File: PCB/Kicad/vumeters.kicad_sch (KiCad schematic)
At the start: 80 parts

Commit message: update elements WIP
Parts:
- D1, D10, D11, D12, D13, D14, D15, D16, D17, D18, D19, D2, D20, D21, D22, D23, D24, D25, D26, D27, D28, D29, D3, D30, D31, D32, D33, D34, D35, D36, D37, D38, D39, D4, D40, D5, D6, D7, D8, D9: renamed from D?; symbol Traktorino-rescue:LED_ALT-Device -> Device:LED_Filled
- gave numbers to parts that had none: 40
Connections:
- net GND: now also D1.1 (K), D10.1 (K), D11.1 (K), D12.1 (K), D13.1 (K), D14.1 (K), D15.1 (K), D16.1 (K), D17.1 (K), D18.1 (K), D19.1 (K), D2.1 (K), D20.1 (K), D21.1 (K), D22.1 (K), D23.1 (K), D24.1 (K), D25.1 (K), D26.1 (K), D27.1 (K), D28.1 (K), D29.1 (K), D3.1 (K), D30.1 (K), D31.1 (K), D32.1 (K), D33.1 (K), D34.1 (K), D35.1 (K), D36.1 (K), D37.1 (K), D38.1 (K), D39.1 (K), D4.1 (K), D40.1 (K), D5.1 (K), D6.1 (K), D7.1 (K), D8.1 (K), D9.1 (K)
- net at R1.2: now also D1.2 (A)
- net at R2.2: now also D2.2 (A)
- net at R3.2: now also D3.2 (A)
- net at R4.2: now also D4.2 (A)
- net at R5.2: now also D5.2 (A)
- net at R6.2: now also D6.2 (A)
- net at R7.2: now also D7.2 (A)
- net at R8.2: now also D8.2 (A)
- net at R16.2: now also D16.2 (A)
- net at R15.2: now also D15.2 (A)
- net at R14.2: now also D14.2 (A)
- net at R13.2: now also D13.2 (A)
- net at R12.2: now also D12.2 (A)
- net at R11.2: now also D11.2 (A)
- net at R10.2: now also D10.2 (A)
- net at R9.2: now also D9.2 (A)
- net at R24.2: now also D24.2 (A)
- net at R23.2: now also D23.2 (A)
- net at R22.2: now also D22.2 (A)
- net at R21.2: now also D21.2 (A)
- net at R20.2: now also D20.2 (A)
- net at R19.2: now also D19.2 (A)
- net at R18.2: now also D18.2 (A)
- net at R17.2: now also D17.2 (A)
- net at R32.2: now also D32.2 (A)
- net at R31.2: now also D31.2 (A)
- net at R30.2: now also D30.2 (A)
- net at R29.2: now also D29.2 (A)
- net at R28.2: now also D28.2 (A)
- net at R27.2: now also D27.2 (A)
- net at R26.2: now also D26.2 (A)
- net at R25.2: now also D25.2 (A)
- net at R40.2: now also D40.2 (A)
- net at R39.2: now also D39.2 (A)
- net at R38.2: now also D38.2 (A)
- net at R37.2: now also D37.2 (A)
- net at R36.2: now also D36.2 (A)
- net at R35.2: now also D35.2 (A)
- net at R34.2: now also D34.2 (A)
- net at R33.2: now also D33.2 (A)

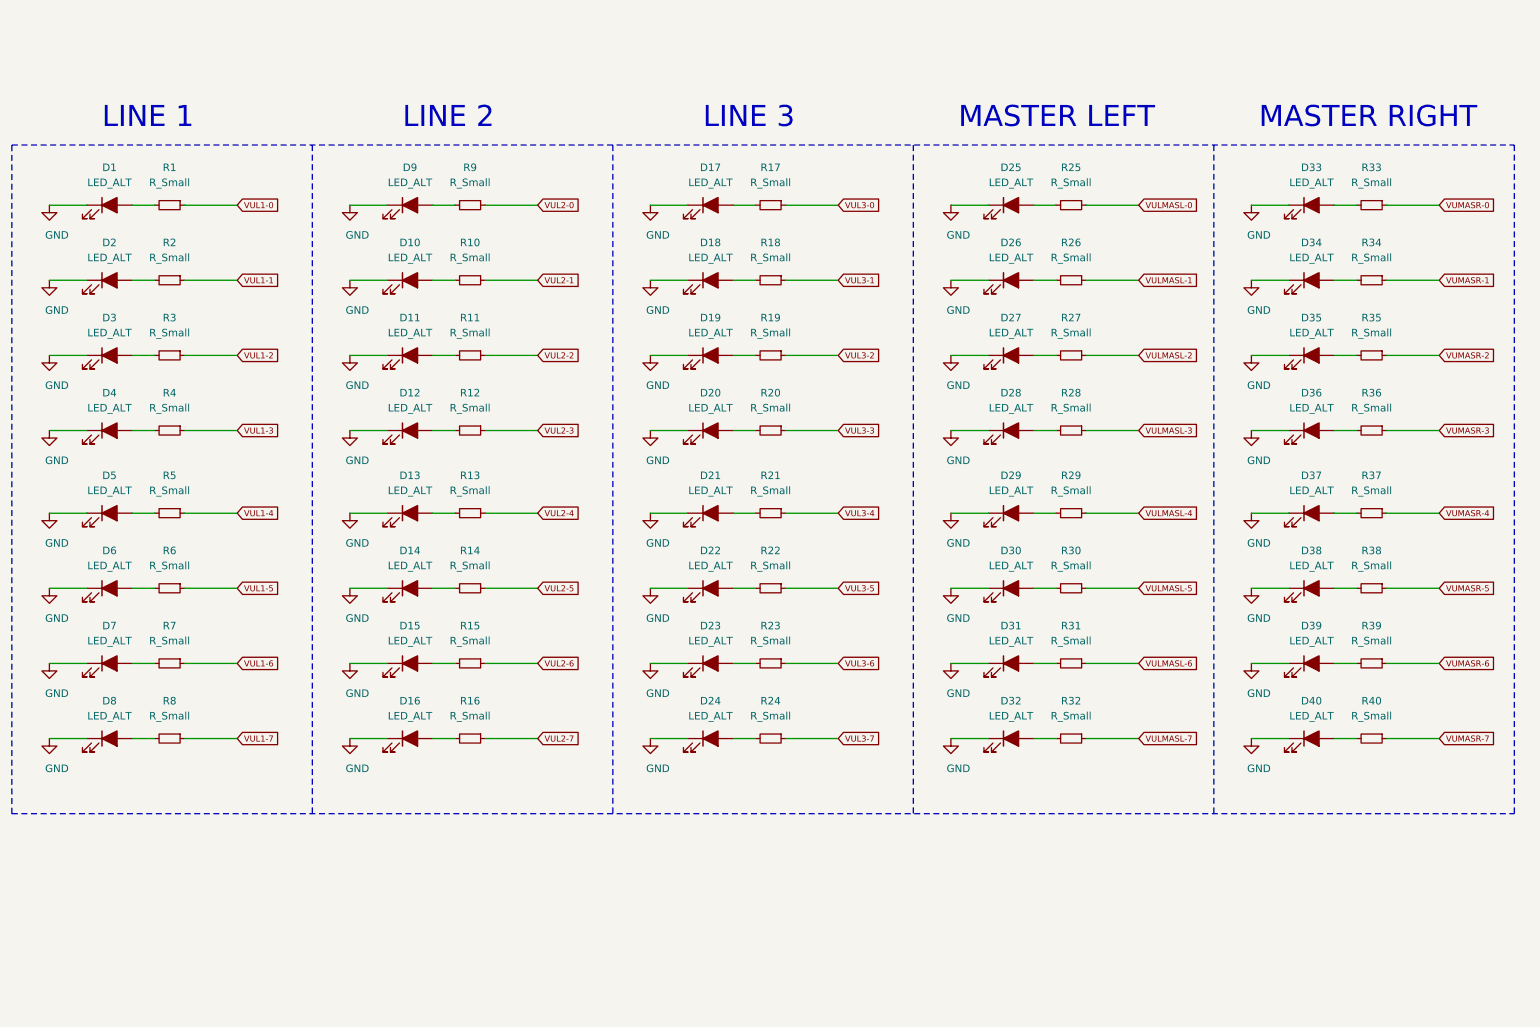
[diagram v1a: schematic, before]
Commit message: progress
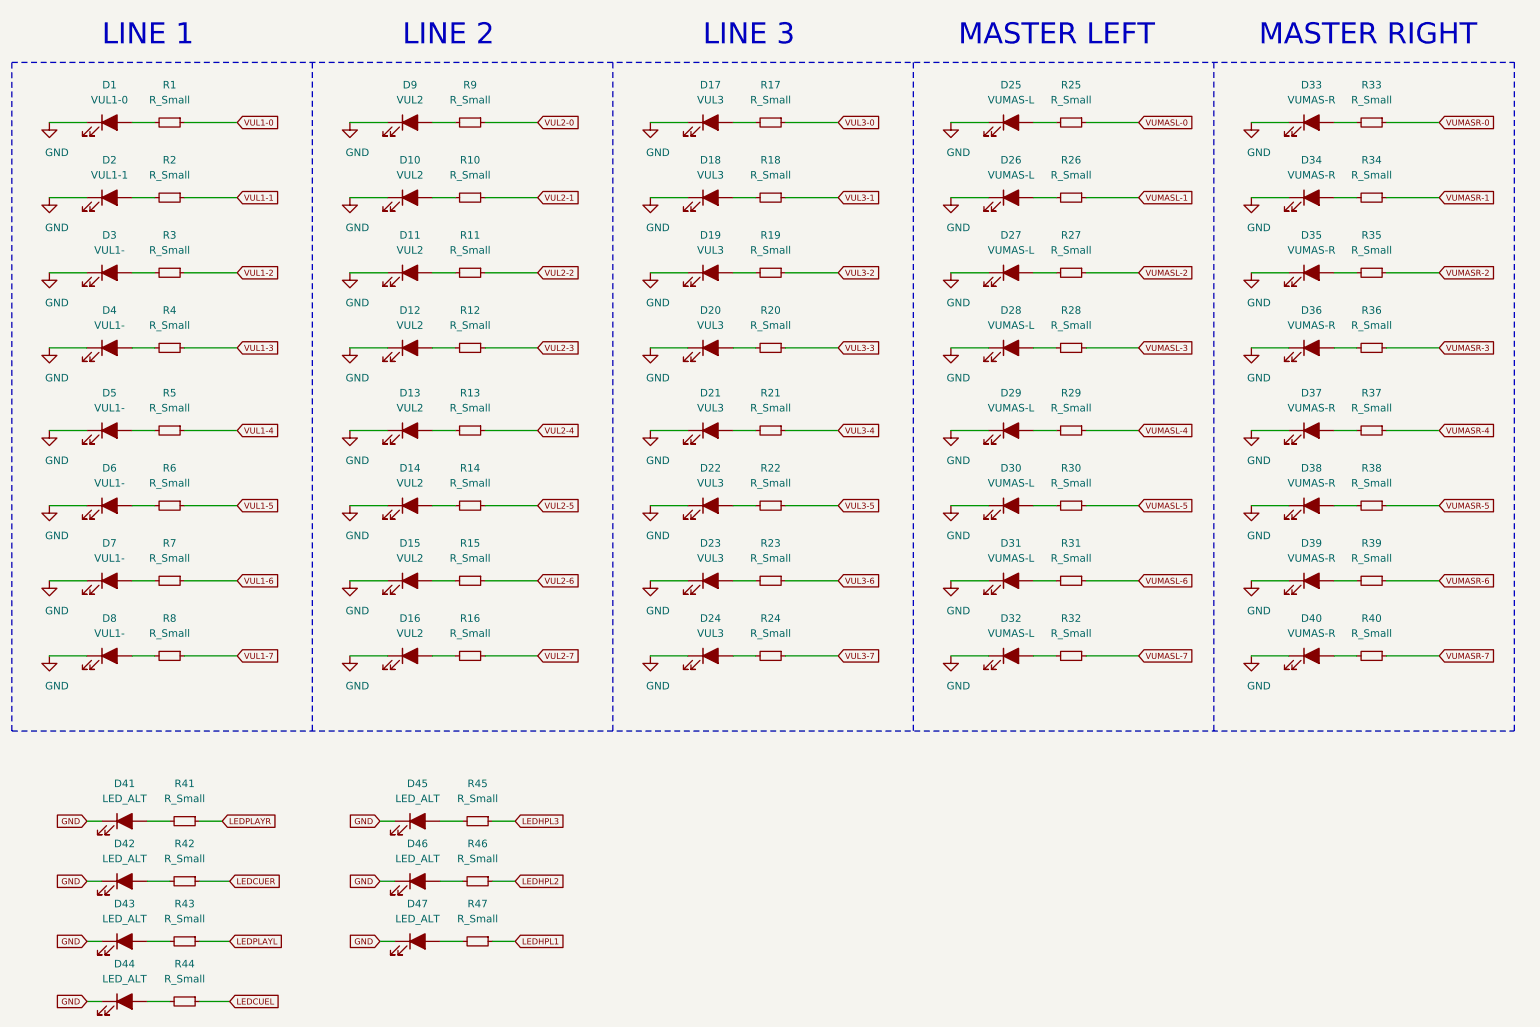
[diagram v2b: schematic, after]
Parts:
- added D41, D42, D43, D44, D45, D46, D47: LED_ALT, LED_THT:LED_Rectangular_W3.0mm_H2.0mm, symbol Device:LED_Filled
- added R41, R42, R43, R44, R45, R46, R47: R_Small, Resistor_THT:R_Axial_DIN0207_L6.3mm_D2.5mm_P7.62mm_Horizontal, symbol Device:R_Small
- D1: value LED_ALT -> VUL1-0; footprint (none) -> LED_THT:LED_Rectangular_W3.0mm_H2.0mm
- D10, D11, D12, D13, D14, D15, D16, D9: value LED_ALT -> VUL2; footprint (none) -> LED_THT:LED_Rectangular_W3.0mm_H2.0mm
- D17, D18, D19, D20, D21, D22, D23, D24: value LED_ALT -> VUL3; footprint (none) -> LED_THT:LED_Rectangular_W3.0mm_H2.0mm
- D2: value LED_ALT -> VUL1-1; footprint (none) -> LED_THT:LED_Rectangular_W3.0mm_H2.0mm
- D25, D26, D27, D28, D29, D30, D31, D32: value LED_ALT -> VUMAS-L; footprint (none) -> LED_THT:LED_Rectangular_W3.0mm_H2.0mm
- D3, D4, D5, D6, D7, D8: value LED_ALT -> VUL1-; footprint (none) -> LED_THT:LED_Rectangular_W3.0mm_H2.0mm
- D33, D34, D35, D36, D37, D38, D39, D40: value LED_ALT -> VUMAS-R; footprint (none) -> LED_THT:LED_Rectangular_W3.0mm_H2.0mm
- R1, R10, R11, R12, R13, R14, R15, R16, R17, R18, R19, R2, R20, R21, R22, R23, R24, R25, R26, R27, R28, R29, R3, R30, R31, R32, R33, R34, R35, R36, R37, R38, R39, R4, R40, R5, R6, R7, R8, R9: footprint (none) -> Resistor_THT:R_Axial_DIN0207_L6.3mm_D2.5mm_P7.62mm_Horizontal
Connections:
- net GND: now also D41.1 (K), D42.1 (K), D43.1 (K), D44.1 (K), D45.1 (K), D46.1 (K), D47.1 (K)
- net VULMASL-0 renamed VUMASL-0
- net VULMASL-1 renamed VUMASL-1
- net VULMASL-2 renamed VUMASL-2
- net VULMASL-3 renamed VUMASL-3
- net VULMASL-4 renamed VUMASL-4
- net VULMASL-5 renamed VUMASL-5
- net VULMASL-6 renamed VUMASL-6
- net VULMASL-7 renamed VUMASL-7
- new net: D44.2 (A), R44.2
- new net: D42.2 (A), R42.2
- new net: D47.2 (A), R47.2
- new net: D45.2 (A), R45.2
- new net: D43.2 (A), R43.2
- new net: D46.2 (A), R46.2
- new net: D41.2 (A), R41.2
- new net LEDCUEL: R44.1
- new net LEDCUER: R42.1
- new net LEDHPL1: R47.1
- new net LEDHPL2: R46.1
- new net LEDHPL3: R45.1
- new net LEDPLAYL: R43.1
- new net LEDPLAYR: R41.1
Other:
- moved on the sheet: D1, D10, D11, D12, D13, D14, D15, D16, D17, D18, D19, D2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
